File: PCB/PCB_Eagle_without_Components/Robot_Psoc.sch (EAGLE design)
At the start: 131 parts

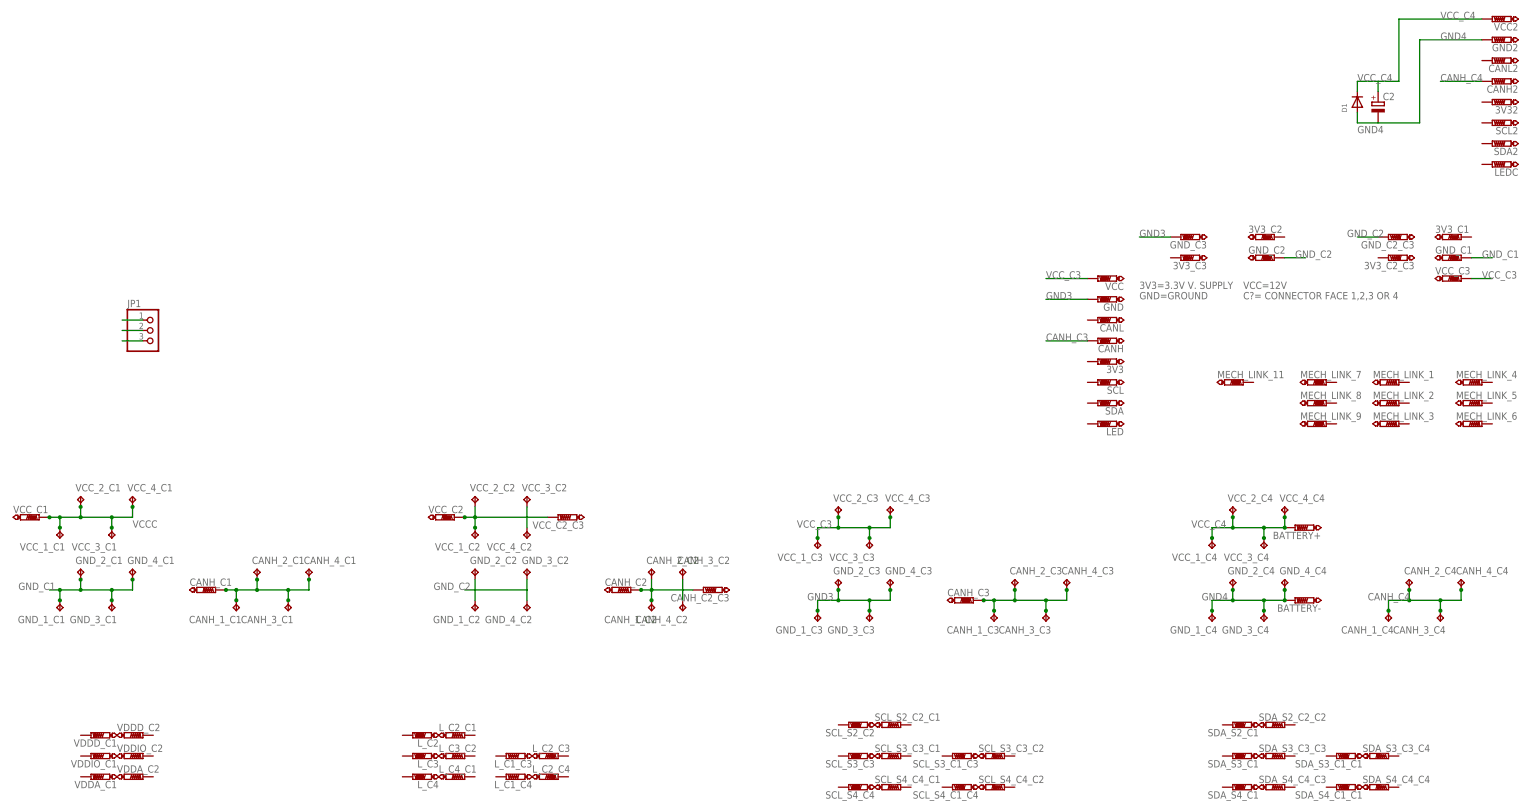
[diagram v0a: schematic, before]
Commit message: 05/May
PCB
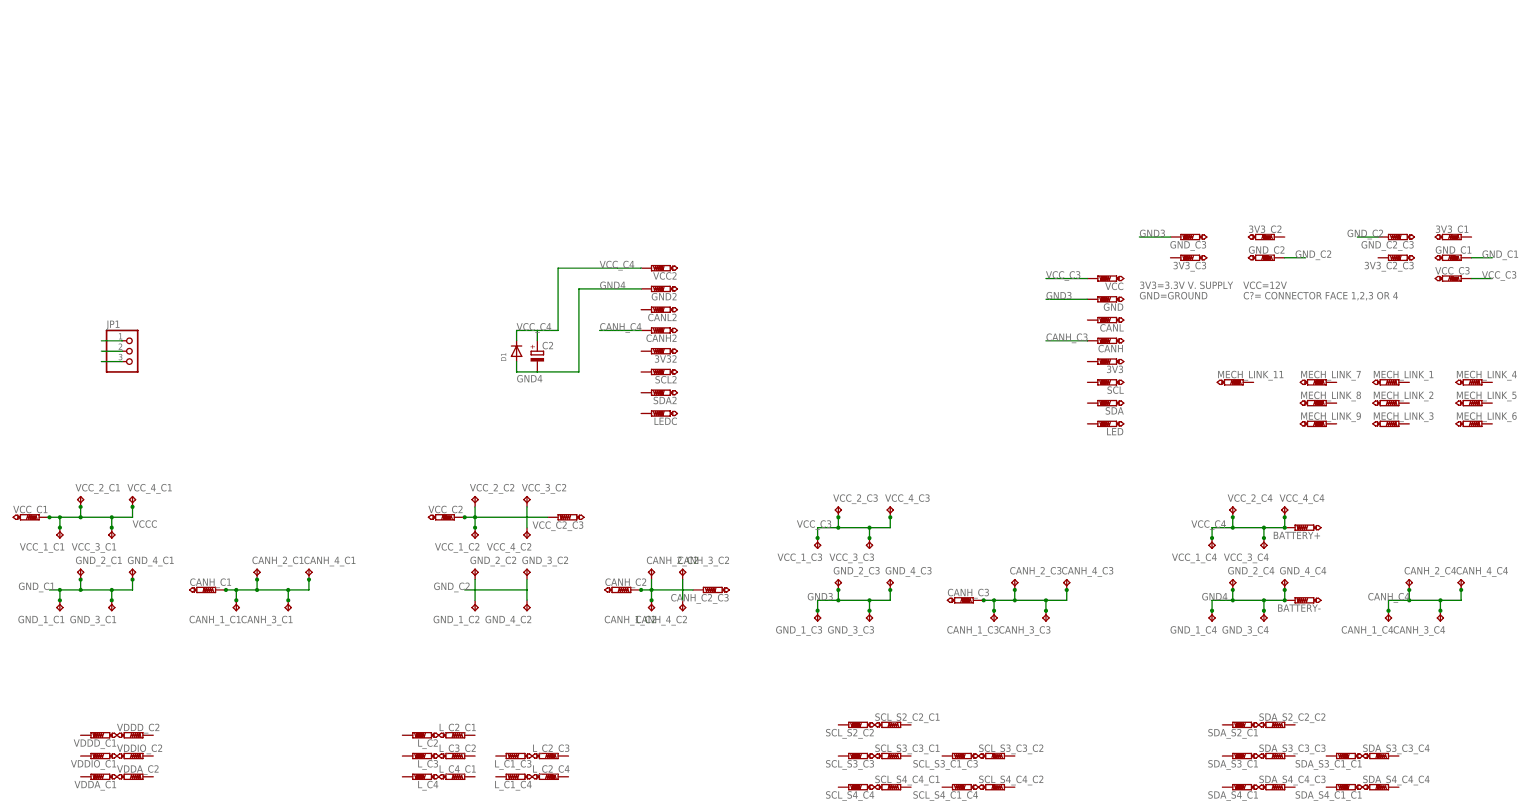
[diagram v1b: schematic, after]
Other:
- note added: "FACE 1 COMPONENT'S"
- moved on the sheet: 3V32, C2, CANH2, CANL2, D1, GND2, JP1, LEDC, SCL2, SDA2, VCC2
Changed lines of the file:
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@@
 <sheet>
 <plain>
-<wire x1="7.62" y1="96.52" x2="7.62" y2="-35.56" width="1.4224" layer="105"/>
-<wire x1="7.62" y1="-35.56" x2="190.5" y2="-35.56" width="1.4224" layer="105"/>
+<wire x1="7.62" y1="-35.56" x2="99.06" y2="-35.56" width="1.4224" layer="105"/>
+<wire x1="99.06" y1="-35.56" x2="190.5" y2="-35.56" width="1.4224" layer="105"/>
 <wire x1="190.5" y1="-35.56" x2="190.5" y2="27.94" width="1.4224" layer="105"/>
-<wire x1="190.5" y1="96.52" x2="7.62" y2="96.52" width="1.4224" layer="105"/>
-<wire x1="190.5" y1="96.52" x2="297.18" y2="96.52" width="1.4224" layer="105"/>
-<wire x1="297.18" y1="96.52" x2="297.18" y2="27.94" width="1.4224" layer="105"/>
+<wire x1="7.62" y1="27.94" x2="99.06" y2="27.94" width="1.4224" layer="105"/>
+<wire x1="99.06" y1="27.94" x2="190.5" y2="27.94" width="1.4224" layer="105"/>
 <wire x1="297.18" y1="27.94" x2="190.5" y2="27.94" width="1.4224" layer="105"/>
-<wire x1="190.5" y1="27.94" x2="190.5" y2="96.52" width="1.4224" layer="105"/>
 <text x="208.28" y="20.32" size="5.08" layer="105">FACE 3 COMPONENT'S</text>
 <wire x1="190.5" y1="-35.56" x2="297.18" y2="-35.56" width="1.4224" layer="105"/>
-<text x="312.42" y="88.9" size="5.08" layer="105">FACE 4 COMPONENT'S</text>
+<text x="111.76" y="17.78" size="5.08" layer="105">FACE 4 COMPONENT'S</text>
 <wire x1="297.18" y1="-7.62" x2="297.18" y2="27.94" width="1.4224" layer="105"/>
 <wire x1="297.18" y1="27.94" x2="396.24" y2="27.94" width="1.4224" layer="105"/>
-<wire x1="396.24" y1="27.94" x2="396.24" y2="96.52" width="1.4224" layer="105"/>
-<wire x1="396.24" y1="96.52" x2="297.18" y2="96.52" width="1.4224" layer="105"/>
 <wire x1="297.18" y1="-35.56" x2="396.24" y2="-35.56" width="1.4224" layer="105"/>
 <wire x1="396.24" y1="-35.56" x2="396.24" y2="-7.62" width="1.4224" layer="105"/>
@@
 <wire x1="297.18" y1="-35.56" x2="297.18" y2="-7.62" width="1.4224" layer="105"/>
 <wire x1="297.18" y1="-7.62" x2="396.24" y2="-7.62" width="1.4224" layer="105"/>
-<wire x1="7.62" y1="-35.56" x2="7.62" y2="-86.36" width="1.4224" layer="105"/>
+<wire x1="7.62" y1="-35.56" x2="7.62" y2="-40.64" width="1.4224" layer="105"/>
+<wire x1="7.62" y1="-40.64" x2="7.62" y2="-86.36" width="1.4224" layer="105"/>
 <wire x1="7.62" y1="-86.36" x2="396.24" y2="-86.36" width="1.4224" layer="105"/>
 <wire x1="396.24" y1="-86.36" x2="396.24" y2="-35.56" width="1.4224" layer="105"/>
@@
 <text x="325.12" y="2.54" size="1.778" layer="95">VCC=12V </text>
 <text x="325.12" y="0" size="1.778" layer="95">C?= CONNECTOR FACE 1,2,3 OR 4</text>
+<text x="17.78" y="17.78" size="5.08" layer="105">FACE 1 COMPONENT'S</text>
+<wire x1="7.62" y1="-35.56" x2="7.62" y2="27.94" width="1.4224" layer="105"/>
+<wire x1="99.06" y1="-35.56" x2="99.06" y2="27.94" width="1.4224" layer="105"/>
 </plain>
 <instances>
@@
 <instance part="SDA" gate="G$1" x="289.56" y="-25.4" rot="R90"/>
 <instance part="LED" gate="G$1" x="289.56" y="-30.48" rot="R90"/>
-<instance part="VCC2" gate="G$1" x="386.08" y="68.58" rot="R90"/>
-<instance part="GND2" gate="G$1" x="386.08" y="63.5" rot="R90"/>
-<instance part="CANL2" gate="G$1" x="386.08" y="58.42" rot="R90"/>
-<instance part="CANH2" gate="G$1" x="386.08" y="53.34" rot="R90"/>
-<instance part="3V32" gate="G$1" x="386.08" y="48.26" rot="R90"/>
-<instance part="SCL2" gate="G$1" x="386.08" y="43.18" rot="R90"/>
-<instance part="SDA2" gate="G$1" x="386.08" y="38.1" rot="R90"/>
-<instance part="LEDC" gate="G$1" x="386.08" y="33.02" rot="R90"/>
-<instance part="C2" gate="G$1" x="358.14" y="48.26"/>
-<instance part="D1" gate="G$1" x="353.06" y="48.26" rot="R90"/>
-<instance part="JP1" gate="A" x="58.42" y="-7.62"/>
+<instance part="VCC2" gate="G$1" x="180.34" y="7.62" rot="R90"/>
+<instance part="GND2" gate="G$1" x="180.34" y="2.54" rot="R90"/>
+<instance part="CANL2" gate="G$1" x="180.34" y="-2.54" rot="R90"/>
+<instance part="CANH2" gate="G$1" x="180.34" y="-7.62" rot="R90"/>
+<instance part="3V32" gate="G$1" x="180.34" y="-12.7" rot="R90"/>
+<instance part="SCL2" gate="G$1" x="180.34" y="-17.78" rot="R90"/>
+<instance part="SDA2" gate="G$1" x="180.34" y="-22.86" rot="R90"/>
+<instance part="LEDC" gate="G$1" x="180.34" y="-27.94" rot="R90"/>
+<instance part="C2" gate="G$1" x="152.4" y="-12.7"/>
+<instance part="D1" gate="G$1" x="147.32" y="-12.7" rot="R90"/>
+<instance part="JP1" gate="A" x="53.34" y="-12.7"/>
 </instances>
 <busses>
@@
 <segment>
 <pinref part="JP1" gate="A" pin="3"/>
-<wire x1="50.8" y1="-10.16" x2="55.88" y2="-10.16" width="0.1524" layer="91"/>
+<wire x1="45.72" y1="-15.24" x2="50.8" y2="-15.24" width="0.1524" layer="91"/>
 </segment>
 </net>
@@
 <segment>
 <pinref part="JP1" gate="A" pin="2"/>
-<wire x1="50.8" y1="-7.62" x2="55.88" y2="-7.62" width="0.1524" layer="91"/>
+<wire x1="45.72" y1="-12.7" x2="50.8" y2="-12.7" width="0.1524" layer="91"/>
 </segment>
 </net>
@@
 </segment>
 <segment>
-<label x="373.38" y="63.5" size="1.778" layer="95"/>
+<label x="167.64" y="2.54" size="1.778" layer="95"/>
 <pinref part="C2" gate="G$1" pin="-"/>
 <pinref part="D1" gate="G$1" pin="A"/>
-<wire x1="353.06" y1="45.72" x2="353.06" y2="43.18" width="0.1524" layer="91"/>
-<wire x1="353.06" y1="43.18" x2="358.14" y2="43.18" width="0.1524" layer="91"/>
-<wire x1="358.14" y1="43.18" x2="368.3" y2="43.18" width="0.1524" layer="91"/>
-<wire x1="368.3" y1="43.18" x2="368.3" y2="63.5" width="0.1524" layer="91"/>
+<wire x1="147.32" y1="-15.24" x2="147.32" y2="-17.78" width="0.1524" layer="91"/>
+<wire x1="147.32" y1="-17.78" x2="152.4" y2="-17.78" width="0.1524" layer="91"/>
+<wire x1="152.4" y1="-17.78" x2="162.56" y2="-17.78" width="0.1524" layer="91"/>
+<wire x1="162.56" y1="-17.78" x2="162.56" y2="2.54" width="0.1524" layer="91"/>
 <pinref part="GND2" gate="G$1" pin="TP"/>
-<wire x1="368.3" y1="63.5" x2="383.54" y2="63.5" width="0.1524" layer="91"/>
-<label x="353.06" y="40.64" size="1.778" layer="95"/>
+<wire x1="162.56" y1="2.54" x2="177.8" y2="2.54" width="0.1524" layer="91"/>
+<label x="147.32" y="-20.32" size="1.778" layer="95"/>
 </segment>
 </net>
@@
 <segment>
 <pinref part="JP1" gate="A" pin="1"/>
-<wire x1="50.8" y1="-5.08" x2="55.88" y2="-5.08" width="0.1524" layer="91"/>
+<wire x1="45.72" y1="-10.16" x2="50.8" y2="-10.16" width="0.1524" layer="91"/>
 </segment>
 </net>
@@
 </segment>
 <segment>
-<label x="373.38" y="68.58" size="1.778" layer="95"/>
+<label x="167.64" y="7.62" size="1.778" layer="95"/>
 <pinref part="C2" gate="G$1" pin="+"/>
-<wire x1="358.14" y1="50.8" x2="358.14" y2="53.34" width="0.1524" layer="91"/>
+<wire x1="152.4" y1="-10.16" x2="152.4" y2="-7.62" width="0.1524" layer="91"/>
 <pinref part="D1" gate="G$1" pin="C"/>
-<wire x1="353.06" y1="50.8" x2="353.06" y2="53.34" width="0.1524" layer="91"/>
-<wire x1="353.06" y1="53.34" x2="358.14" y2="53.34" width="0.1524" layer="91"/>
+<wire x1="147.32" y1="-10.16" x2="147.32" y2="-7.62" width="0.1524" layer="91"/>
+<wire x1="147.32" y1="-7.62" x2="152.4" y2="-7.62" width="0.1524" layer="91"/>
 <pinref part="VCC2" gate="G$1" pin="TP"/>
-<wire x1="383.54" y1="68.58" x2="363.22" y2="68.58" width="0.1524" layer="91"/>
-<wire x1="363.22" y1="68.58" x2="363.22" y2="53.34" width="0.1524" layer="91"/>
-<wire x1="363.22" y1="53.34" x2="358.14" y2="53.34" width="0.1524" layer="91"/>
-<label x="353.06" y="53.34" size="1.778" layer="95"/>
+<wire x1="177.8" y1="7.62" x2="157.48" y2="7.62" width="0.1524" layer="91"/>
+<wire x1="157.48" y1="7.62" x2="157.48" y2="-7.62" width="0.1524" layer="91"/>
+<wire x1="157.48" y1="-7.62" x2="152.4" y2="-7.62" width="0.1524" layer="91"/>
+<label x="147.32" y="-7.62" size="1.778" layer="95"/>
 </segment>
 </net>
@@
 </segment>
 <segment>
-<wire x1="383.54" y1="53.34" x2="373.38" y2="53.34" width="0.1524" layer="91"/>
-<label x="373.38" y="53.34" size="1.778" layer="95"/>
+<wire x1="177.8" y1="-7.62" x2="167.64" y2="-7.62" width="0.1524" layer="91"/>
+<label x="167.64" y="-7.62" size="1.778" layer="95"/>
 <pinref part="CANH2" gate="G$1" pin="TP"/>
 </segment>
